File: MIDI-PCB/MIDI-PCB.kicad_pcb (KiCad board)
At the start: 2 copper layers, 43 parts, among them J1 display, J2 Keypad, J3 Rotary encoder, J4 Conn_01x06, J5 Conn_01x06, J6 Conn_01x06, J7 Conn_01x12, J8 Conn_01x12, J9 Conn_01x12, SW1 SW_Push, SW2 SW_Push, U1 XIAO-RP2040-SMD

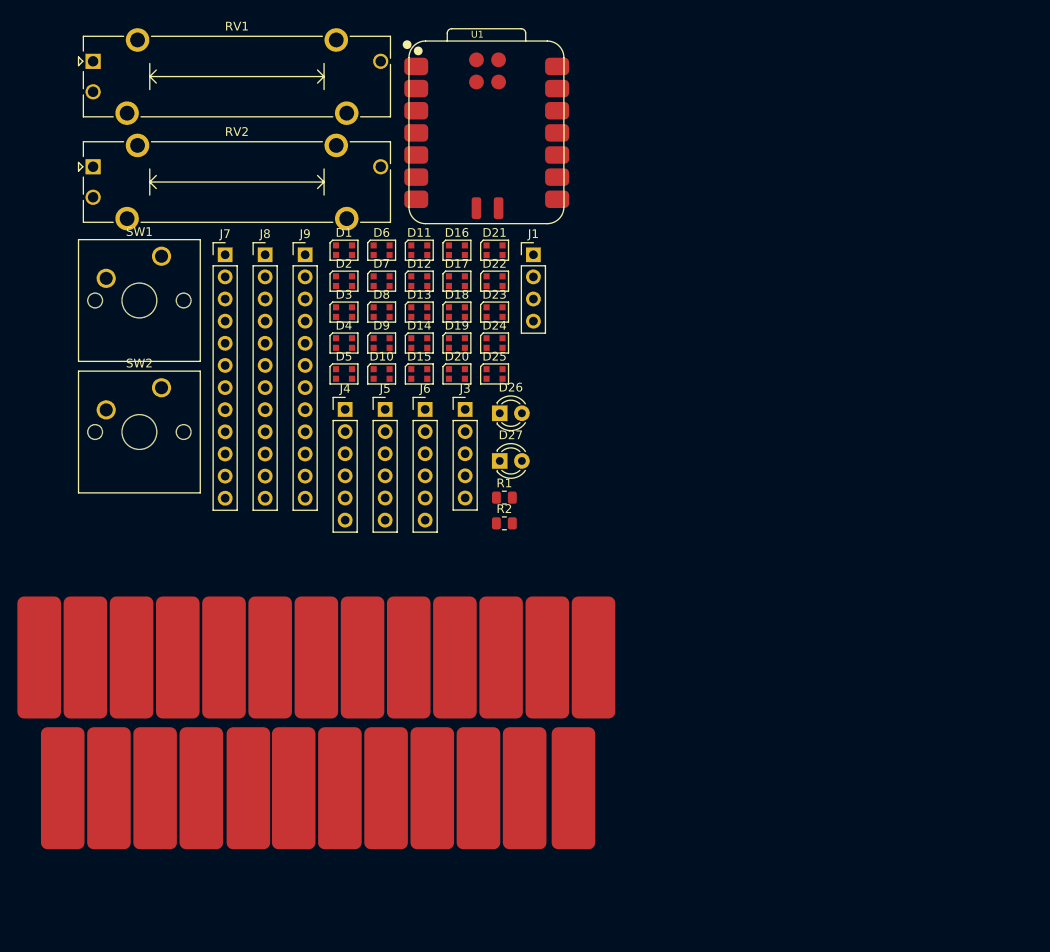
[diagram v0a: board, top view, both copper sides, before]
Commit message: YAY
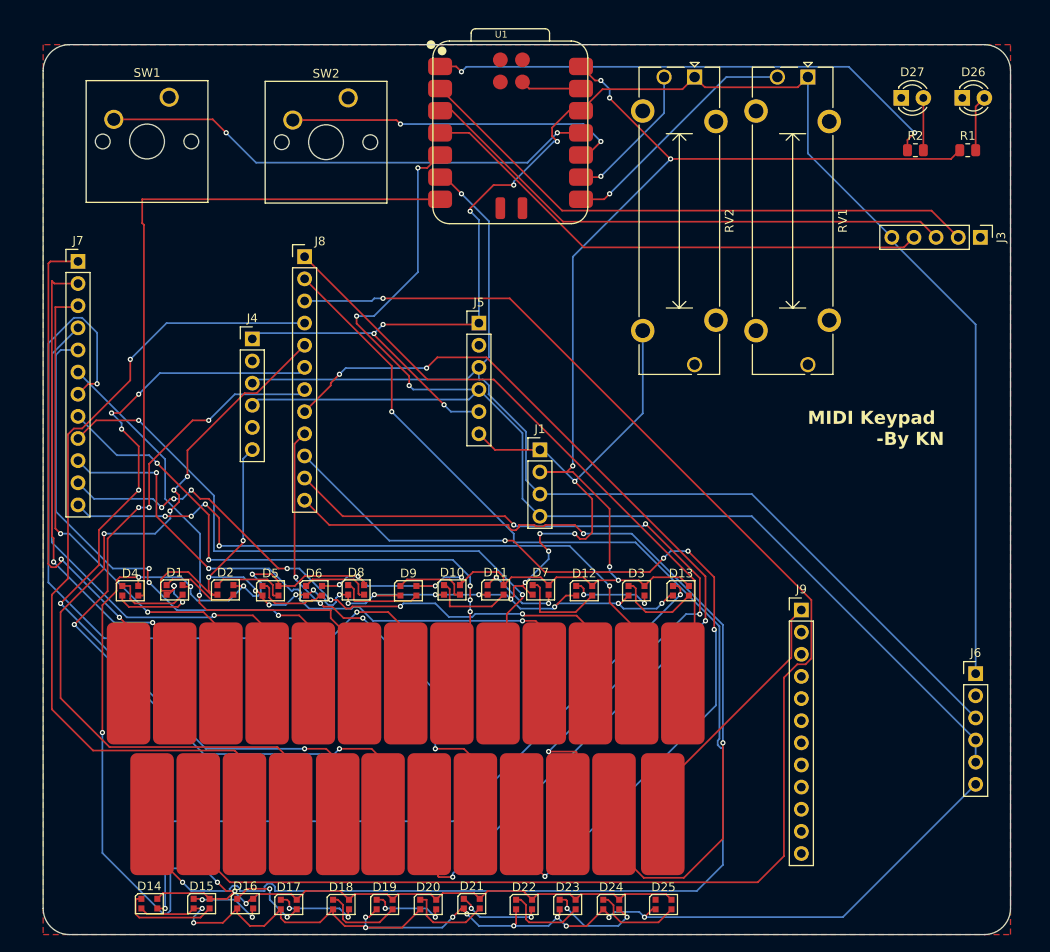
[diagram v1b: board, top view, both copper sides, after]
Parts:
- added ?: LOGO, Rocket_solder:orph, B.Cu at (197.0, 148.0)
- added ?: LOGO, art:1, B.Cu at (183.0, 114.0)
- added ?: LOGO, Rocket_solder2:kitty, B.Cu at (146.0, 149.0)
- added G***: LOGO, art:musicig, B.Cu at (153.6, 90.4)
- added G***: LOGO, art:cool cat, B.Cu at (117.0, 122.0)
- moved RV1 82.0 mm to (187.8, 73.6), turned to -90 degrees
- moved D16 78.8 mm to (123.2, 168.4)
- moved D21 75.0 mm to (149.2, 168.4)
- moved D17 74.1 mm to (128.2, 168.6)
- moved D22 71.6 mm to (155.2, 168.6)
- moved D14 71.4 mm to (112.2, 168.4)
- moved J6 70.1 mm to (207.0, 142.1)
- moved J9 70.0 mm to (187.0, 134.8)
- moved RV2 69.8 mm to (174.8, 73.6), turned to -90 degrees
- moved D18 69.3 mm to (134.2, 168.6)
- moved D23 68.5 mm to (160.2, 168.6)
- moved R1 66.4 mm to (206.1, 82.0)
- moved D24 65.8 mm to (165.2, 168.6)
- moved D15 65.7 mm to (118.2, 168.4)
- moved D19 65.0 mm to (139.2, 168.6)
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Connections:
- D2 pad 1: unconnected-(D2-DOUT-Pad1) -> Net-(D2-DOUT)
- D5 pad 3: unconnected-(D5-DIN-Pad3) -> Net-(D2-DOUT)
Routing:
- net +5V: track 0.00 -> 325.2 mm, vias 0 -> 18
- net GND: track 0.00 -> 308.5 mm, vias 0 -> 34
- net KEY_15: track 0.00 -> 182.8 mm, vias 0 -> 1
- net +3V3: track 0.00 -> 180.6 mm, vias 0 -> 6
- net KEY_14: track 0.00 -> 175.4 mm, vias 0 -> 2
- net SDA: track 0.00 -> 150.3 mm, vias 0 -> 3
- net SCL: track 0.00 -> 130.1 mm, vias 0 -> 1
- net KEY_20: track 0.00 -> 119.7 mm, vias 0 -> 4
- net KEY_22: track 0.00 -> 110.3 mm, vias 0 -> 5
- net KEY_24: track 0.00 -> 103.8 mm, vias 0 -> 2
- net KEY_16: track 0.00 -> 92.1 mm, vias 0 -> 1
- net KEY_18: track 0.00 -> 91.8 mm, vias 0 -> 6
- net KEY_7: track 0.00 -> 90.6 mm, vias 0 -> 2
- net KEY_19: track 0.00 -> 87.9 mm, vias 0 -> 5
- net KEY_17: track 0.00 -> 87.6 mm, vias 0 -> 4
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- added copper zone on F.Cu, net GND
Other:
- board outline added: 111 x 102.1 mm
- board text added: "MIDI Keypad -By KN"
